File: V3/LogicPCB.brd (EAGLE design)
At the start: 171.9 x 151.6 mm, 65 parts, among them CON1 CUBE_ORANGE_, CON11 CON-4P-JST-XA, CON13 CON-6P-JST-XA, CON14 PINHEAD_1X04-2.54, CON15 CON-4P-JST-XA, CON17 CON-4P-JST-XA, CON18 CON-6P-JST-XA, CON19 USB-TYPE-C-VERT-PROD, CON2 CON-4P-JST-XA, CON20 PINHEAD_1X06-2.54, CON21 CON-4P-JST-XA, CON22 CON-4P-JST-XA, CON23 CON-4P-JST-XA, CON24 CON-4P-JST-XA, CON25 CON-4P-JST-XA, CON26 CON-4P-JST-XA, CON27 CON-4P-JST-XA, CON28 CON-4P-JST-XA, CON29 CON-4P-JST-XA, CON3 PINHEAD_1X04-2.54, CON30 CON-4P-JST-XA, CON32 CON-4P-JST-XA, CON35 CON-12P-JST-XA, CON4 CON-2P-JST-XA, CON5 CON-6P-JST-XA, CON6 CON-4P-JST-XA, CON7 PINHEAD_1X06-2.54, CON8 PINHEAD_1X08-2.54, CON9 PINHEAD_1X12-2.54, IC5 AOZ1280, M1 05G_ETHERNET_SWITCH, M2 05G_ETHERNET_SWITCH, Q1 IRLML0030, T1 H1102NL, T2 H1102NL, T3 H1102NL, T4 H1102NL

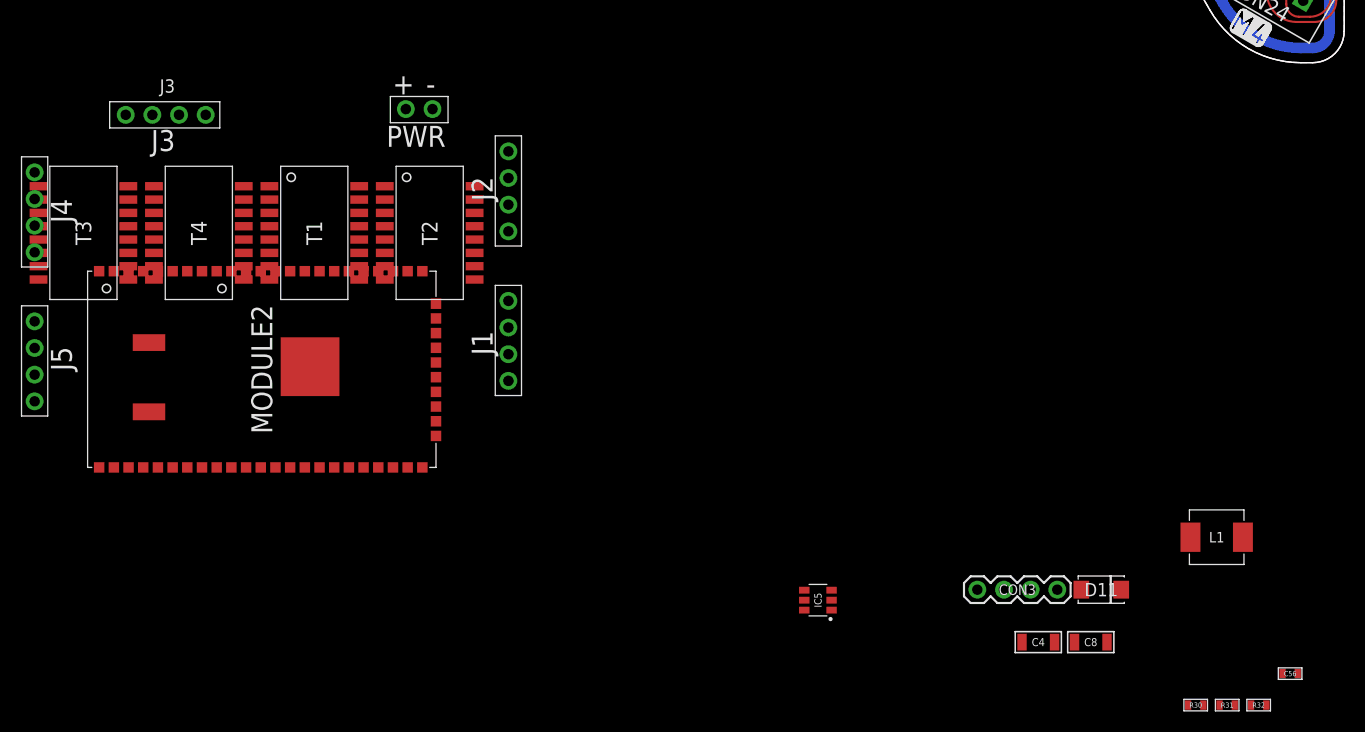
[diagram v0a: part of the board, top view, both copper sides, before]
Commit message: V3 finished
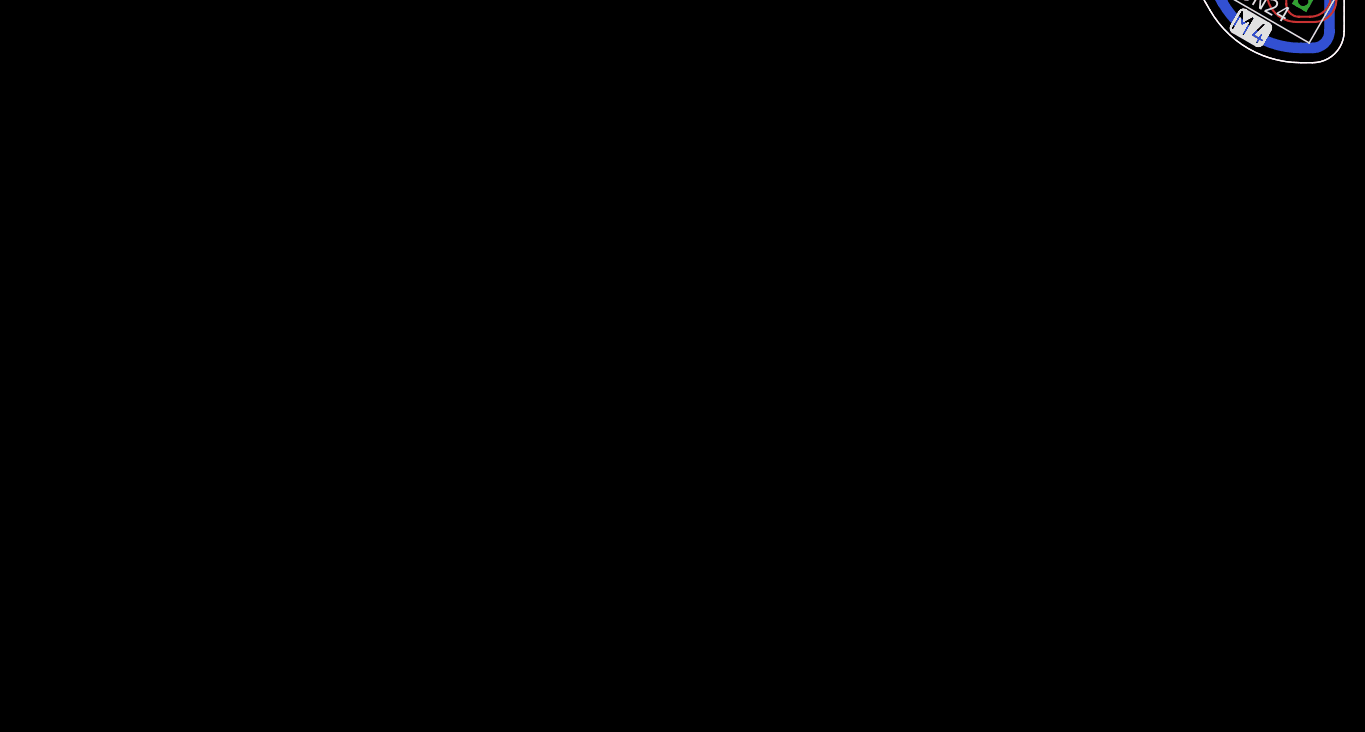
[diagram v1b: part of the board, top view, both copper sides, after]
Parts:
- removed C4: 10u, rc:C1206
- removed C56: 10n, rc:C0603
- removed C8: 47u, rc:C1206
- removed CON3: PINHEAD_1X04-2.54, pinhead:1X04-PTH-2.54
- removed D11: SS34, Diodes:DO-214AC(SMA)
- removed IC5: AOZ1280, dc-dc:SOT23-6
- removed L1: 3.3uH, power_inductors:IHLP-2020BZ-01
- removed M2: 05G_ETHERNET_SWITCH, ali_modules:05G_ETH_SWITCH
- removed MODULE2: HLK-7688A, ali_modules:HLK-7688A
- removed R30, R32: 51K, rc:R0603
- removed R31: 16K, rc:R0603
- removed T1, T2, T3, T4: H1102NL, misc:H1102
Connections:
- removed net CAM_RX+: T1.9
- removed net CAM_TX+: T1.14
- removed net CAM_TX-: T1.16
- removed net CAN_RX-: T1.11
- removed net HLK_RX0: MODULE2.32
- removed net HLK_RX1: MODULE2.16
- removed net HLK_TX0: MODULE2.31
- removed net HLK_TX1: MODULE2.15
- removed net LINK0: MODULE2.13
- removed net LINK1: MODULE2.12
- removed net LINK2: MODULE2.11
- removed net LINK4: MODULE2.9
- removed net LINK_RX+: T4.9
- removed net LINK_RX-: T4.11
- removed net LINK_TX+: T4.14
- removed net LINK_TX-: T4.16
- removed net N$88: C56.2, IC5.1
- removed net N$90: IC5.3, R30.1, R31.1
- removed net N$91: IC5.4, R32.1
- removed net P0_RX+: MODULE2.34, T2.3
- removed net P0_RX-: MODULE2.35, T2.1
- removed net P0_TX+: MODULE2.36, T2.8
- removed net P0_TX-: MODULE2.37, T2.6
- removed net P1_RX+: MODULE2.40, T1.8
- removed net P1_RX-: MODULE2.41, T1.6
- removed net P1_TX+: MODULE2.38, T1.3
- removed net P1_TX-: MODULE2.39, T1.1
- removed net P2_RX+: MODULE2.42, T4.8
- removed net P2_RX-: MODULE2.43, T4.6
- removed net P2_TX+: MODULE2.44, T4.3
- removed net P2_TX-: MODULE2.45, T4.1
- removed net P4_RX+: MODULE2.50, T3.8
- removed net P4_RX-: MODULE2.51, T3.6
- removed net P4_TX+: MODULE2.52, T3.3
- removed net P4_TX-: MODULE2.53, T3.1
- removed net PL_ETH_RX+: T3.11
- removed net PL_ETH_RX-: T3.9
- removed net PL_ETH_TX+: T3.16
- removed net PL_ETH_TX-: T3.14
- removed net SW: C56.1, D11.C, IC5.6, L1.P$1
- removed net USB_DM: CON3.4, MODULE2.55
- removed net USB_DP: CON3.3, MODULE2.54
- removed net VDD_3V3: C8.P$1, L1.P$2, MODULE2.2, MODULE2.3, R30.2
- net GND: no longer C4.P$1, C8.P$2, CON3.1, D11.A, IC5.2, MODULE2.1, MODULE2.21, MODULE2.23, MODULE2.4, MODULE2.56, MODULE2.P$1, MODULE2.P$2, MODULE2.P$3, R31.2
- net VDD_12V: no longer C4.P$2, CON3.2, IC5.5, R32.2
